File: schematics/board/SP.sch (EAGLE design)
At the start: 33 parts

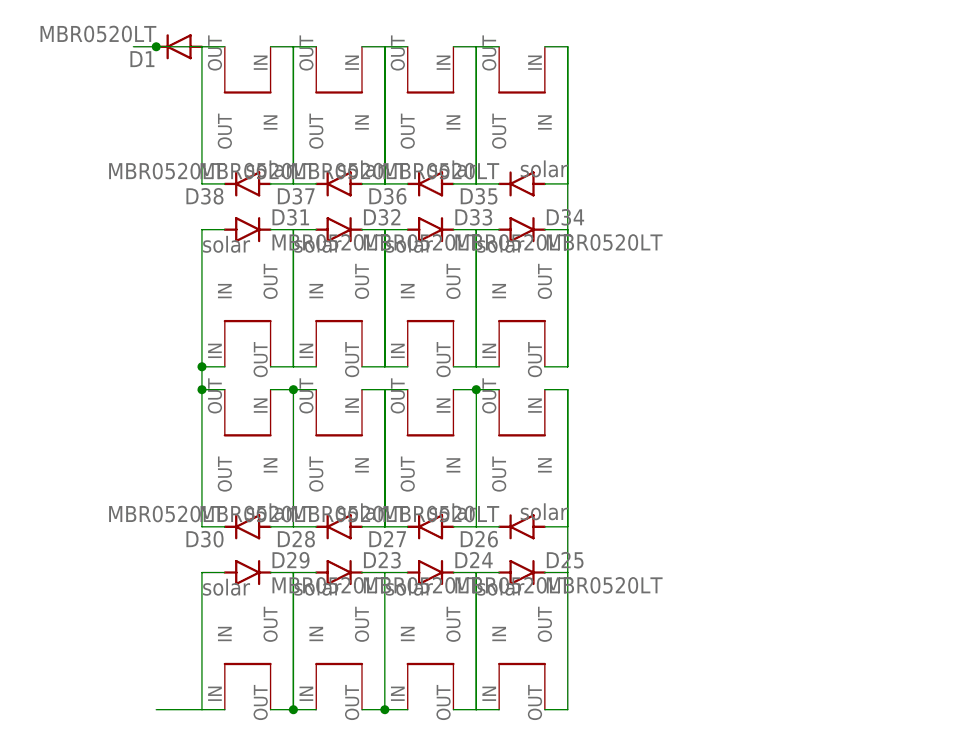
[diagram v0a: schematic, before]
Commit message: Плата СБ
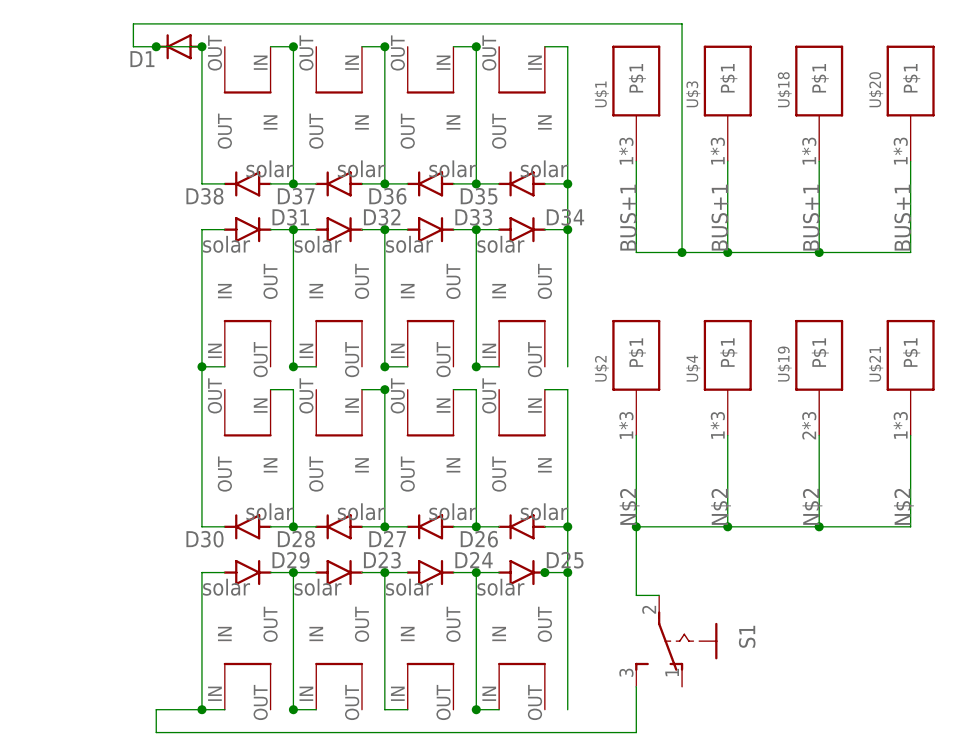
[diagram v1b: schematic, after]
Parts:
- added S1: (no value), CanCubeSat:255SB
- added U$1, U$2, U$20, U$21: KCONNECT--, CanCubeSat:KCONNECT--
- added U$18, U$3, U$4: KCONNECT4, CanCubeSat:KCONNECT4
- added U$19: KCONNECT1, CanCubeSat:KCONNECT1
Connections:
- removed net N$17: D24.C
- removed net N$18: D25.A
- removed net N$20: D26.A
- removed net N$23: D27.C
- removed net N$24: D28.A
- removed net N$26: D29.A
- removed net N$27: D29.C
- removed net N$29: SOL1.IN
- removed net N$30: D1.C, SOL16.OUT
- removed net N$31: D31.C
- removed net N$32: D32.A
- removed net N$33: D32.C
- removed net N$34: D33.A
- removed net N$35: D33.C
- removed net N$36: D34.A
- removed net N$37: D34.C
- removed net N$38: D35.A
- removed net N$39: D35.C
- removed net N$40: D36.A
- removed net N$41: D36.C
- removed net N$42: D37.A
- removed net N$43: D37.C
- removed net N$44: D38.A
- removed net N$45: D1.A, D38.C
- new net BUS+1: D1.A, D1.C, D38.C, U$1.P$1, U$18.P$1, U$20.P$1, U$3.P$1
- new net BUS-1: D29.A, S1.S, SOL1.IN
- new net N$2: S1.P, U$19.P$1, U$2.P$1, U$21.P$1, U$4.P$1
- net N$1: now also D29.C; no longer SOL1.OUT
- net N$10: now also D32.C, D33.A; no longer SOL10.OUT
- net N$11: now also D33.C, D34.A; no longer SOL11.OUT
- net N$12: now also D34.C, D35.A; no longer SOL12.OUT
- net N$13: now also D35.C, D36.A; no longer SOL13.OUT
- net N$14: now also D36.C, D37.A; no longer SOL14.OUT
- net N$15: now also D37.C, D38.A; no longer SOL15.OUT
- net N$16: no longer SOL2.OUT
- net N$19: now also D26.A; no longer SOL4.OUT
- net N$22: no longer SOL5.OUT
- net N$28: no longer SOL7.OUT
- net N$3: now also D24.C, D25.A; no longer SOL3.OUT
- net N$6: now also D27.C, D28.A; no longer SOL6.OUT
- net N$8: no longer SOL8.OUT
- net N$9: now also D31.C, D32.A; no longer SOL9.OUT
